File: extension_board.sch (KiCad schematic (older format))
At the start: 39 parts, among them CN1 Conn_02x20_Odd_Even, J1 Screw_Terminal_01x02, J2 Conn_01x02, J3 Conn_01x02, J4 Conn_01x02, J5 Conn_02x03_Odd_Even, J6 Conn_01x02, J7 Conn_02x14_Odd_Even, J8 Conn_02x10_Odd_Even, J9 Conn_02x19_Odd_Even, U1 LM334Z, U2 LM334Z, U3 LM334Z, U4 LM334Z

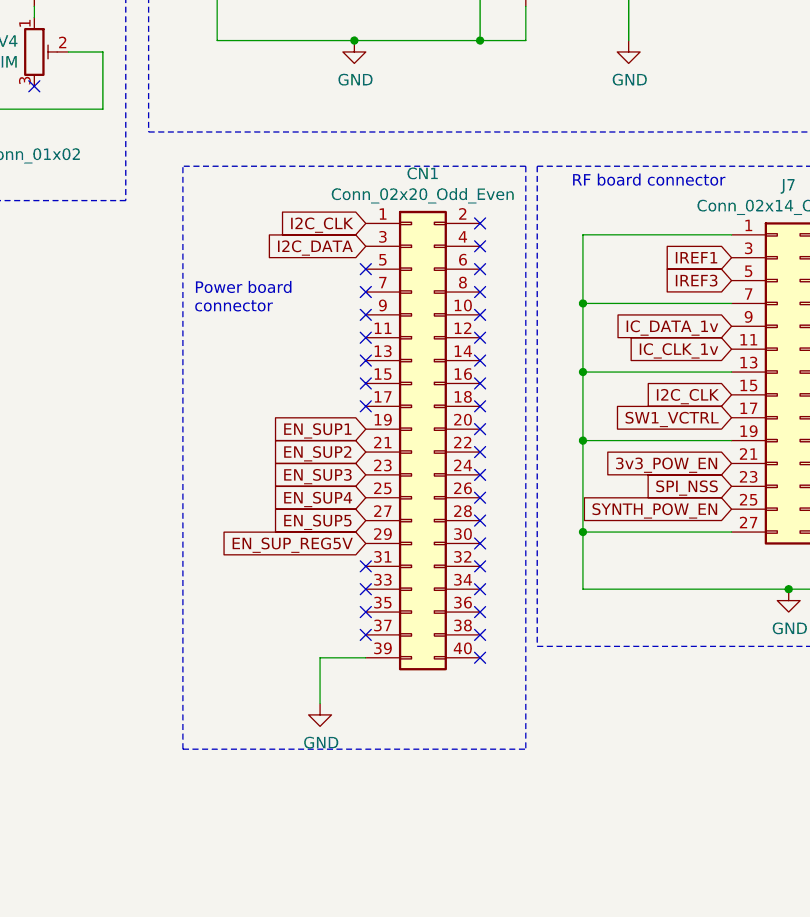
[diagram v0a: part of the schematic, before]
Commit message: gerber files and final files
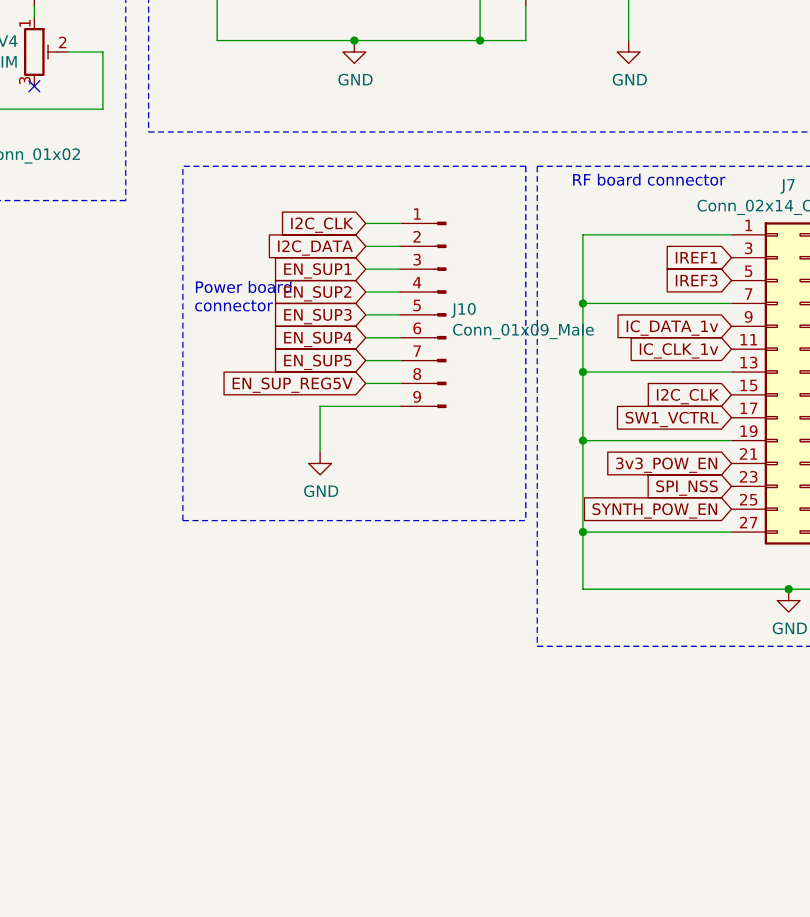
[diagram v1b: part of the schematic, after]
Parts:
- removed CN1: Conn_02x20_Odd_Even, Connector_PinHeader_2.54mm:PinHeader_2x20_P2.54mm_Vertical_SMD, symbol Connector_Generic:Conn_02x20_Odd_Even
- added J10: Conn_01x09_Male, Connector_PinHeader_2.54mm:PinHeader_1x09_P2.54mm_Vertical_SMD_Pin1Left, symbol Connector:Conn_01x09_Male
- J2, J3, J4, J6: footprint Connector_PinHeader_2.54mm:PinHeader_2x01_P2.54mm_Vertical_SMD -> Connector_PinHeader_2.54mm:PinHeader_1x02_P2.54mm_Vertical
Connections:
- net EN_SUP1: now also J10.3 (Pin_3)
- net EN_SUP2: now also J10.4 (Pin_4)
- net EN_SUP3: now also J10.5 (Pin_5)
- net EN_SUP4: now also J10.6 (Pin_6)
- net EN_SUP5: now also J10.7 (Pin_7)
- net EN_SUP_REG5V: now also J10.8 (Pin_8)
- net GND: now also J10.9 (Pin_9)
- net I2C_CLK: now also J10.1 (Pin_1)
- net I2C_DATA: now also J10.2 (Pin_2)
- no-connect marks 58 -> 27
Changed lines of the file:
@@
 1K pot, \nRectangular (3.65mm x 3.00mm x 1.70mm H), \ntop adjust\n
 NoConn ~ 4850 1650
-$Comp
-L Connector_Generic:Conn_02x20_Odd_Even CN1
-U 1 1 6052AEFD
-P 8400 4750
-F 0 "CN1" H 8450 5867 50  0000 C CNN
-F 1 "Conn_02x20_Odd_Even" H 8450 5776 50  0000 C CNN
-F 2 "Connector_PinHeader_2.54mm:PinHeader_2x20_P2.54mm_Vertical_SMD" H 8400 4750 50  0001 C CNN
-F 3 "~" H 8400 4750 50  0001 C CNN
-	1    8400 4750
-	1    0    0    -1
-$EndComp
 Text GLabel 8200 3950 0    50   Input ~ 0
 I2C_DATA
 Text GLabel 8200 3850 0    50   Input ~ 0
 I2C_CLK
-NoConn ~ 8200 4050
-NoConn ~ 8200 4150
-NoConn ~ 8200 4250
-NoConn ~ 8200 4350
-NoConn ~ 8200 4450
-NoConn ~ 8200 4550
-NoConn ~ 8200 4650
-Text GLabel 8200 4750 0    50   Input ~ 0
+Text GLabel 8200 4050 0    50   Input ~ 0
 EN_SUP1
-Text GLabel 8200 4850 0    50   Input ~ 0
+Text GLabel 8200 4150 0    50   Input ~ 0
 EN_SUP2
-Text GLabel 8200 4950 0    50   Input ~ 0
+Text GLabel 8200 4250 0    50   Input ~ 0
 EN_SUP3
-Text GLabel 8200 5050 0    50   Input ~ 0
+Text GLabel 8200 4350 0    50   Input ~ 0
 EN_SUP4
-Text GLabel 8200 5150 0    50   Input ~ 0
+Text GLabel 8200 4450 0    50   Input ~ 0
 EN_SUP5
-Text GLabel 8200 5250 0    50   Input ~ 0
+Text GLabel 8200 4550 0    50   Input ~ 0
 EN_SUP_REG5V
-NoConn ~ 8200 5350
-NoConn ~ 8200 5450
-NoConn ~ 8200 5550
-NoConn ~ 8200 5650
-Wire Wire Line
-	8000 5750 8000 5950
-Wire Wire Line
-	8000 5750 8200 5750
+Wire Wire Line
+	8000 4650 8000 4850
 $Comp
 L power:GND #PWR08
 U 1 1 60545C1E
-P 8000 5950
-F 0 "#PWR08" H 8000 5700 50  0001 C CNN
-F 1 "GND" H 8005 5777 50  0000 C CNN
-F 2 "" H 8000 5950 50  0001 C CNN
-F 3 "" H 8000 5950 50  0001 C CNN
-	1    8000 5950
-	1    0    0    -1
-$EndComp
-NoConn ~ 8700 3850
-NoConn ~ 8700 3950
-NoConn ~ 8700 4050
-NoConn ~ 8700 4150
-NoConn ~ 8700 4250
-NoConn ~ 8700 4350
-NoConn ~ 8700 4450
-NoConn ~ 8700 4550
-NoConn ~ 8700 4650
-NoConn ~ 8700 4750
-NoConn ~ 8700 4850
-NoConn ~ 8700 4950
-NoConn ~ 8700 5050
-NoConn ~ 8700 5150
-NoConn ~ 8700 5250
-NoConn ~ 8700 5350
-NoConn ~ 8700 5450
-NoConn ~ 8700 5550
-NoConn ~ 8700 5650
-NoConn ~ 8700 5750
+P 8000 4850
+F 0 "#PWR08" H 8000 4600 50  0001 C CNN
+F 1 "GND" H 8005 4677 50  0000 C CNN
+F 2 "" H 8000 4850 50  0001 C CNN
+F 3 "" H 8000 4850 50  0001 C CNN
+	1    8000 4850
+	1    0    0    -1
+$EndComp
 Connection ~ 4350 1750
 Wire Wire Line
@@
 Wire Wire Line
 	4350 750  4350 650
-Wire Notes Line
-	8900 3600 8900 6150
-Wire Notes Line
-	7400 6150 7400 3600
 Text Notes 7450 4250 0    50   ~ 0
 Power board \nconnector
@@
 Wire Notes Line
 	8950 3600 11100 3600
-Wire Notes Line
-	7400 6150 8900 6150
 Text GLabel 3850 2250 0    50   Input ~ 0
 VDD
@@
 F 0 "J3" H 4630 1892 50  0000 L CNN
 F 1 "Conn_01x02" H 4630 1801 50  0000 L CNN
-F 2 "Connector_PinHeader_2.54mm:PinHeader_2x01_P2.54mm_Vertical_SMD" H 4550 1900 50  0001 C CNN
+F 2 "Connector_PinHeader_2.54mm:PinHeader_1x02_P2.54mm_Vertical" H 4550 1900 50  0001 C CNN
 F 3 "~" H 4550 1900 50  0001 C CNN
 	1    4550 1900
@@
 F 0 "J2" H 4130 3442 50  0000 L CNN
 F 1 "Conn_01x02" H 4130 3351 50  0000 L CNN
-F 2 "Connector_PinHeader_2.54mm:PinHeader_2x01_P2.54mm_Vertical_SMD" H 4050 3450 50  0001 C CNN
+F 2 "Connector_PinHeader_2.54mm:PinHeader_1x02_P2.54mm_Vertical" H 4050 3450 50  0001 C CNN
 F 3 "~" H 4050 3450 50  0001 C CNN
 	1    4050 3450
@@
 F 0 "J4" H 5380 3442 50  0000 L CNN
 F 1 "Conn_01x02" H 5380 3351 50  0000 L CNN
-F 2 "Connector_PinHeader_2.54mm:PinHeader_2x01_P2.54mm_Vertical_SMD" H 5300 3450 50  0001 C CNN
+F 2 "Connector_PinHeader_2.54mm:PinHeader_1x02_P2.54mm_Vertical" H 5300 3450 50  0001 C CNN
 F 3 "~" H 5300 3450 50  0001 C CNN
 	1    5300 3450
@@
 F 0 "J6" H 6530 3442 50  0000 L CNN
 F 1 "Conn_01x02" H 6530 3351 50  0000 L CNN
-F 2 "Connector_PinHeader_2.54mm:PinHeader_2x01_P2.54mm_Vertical_SMD" H 6450 3450 50  0001 C CNN
+F 2 "Connector_PinHeader_2.54mm:PinHeader_1x02_P2.54mm_Vertical" H 6450 3450 50  0001 C CNN
 F 3 "~" H 6450 3450 50  0001 C CNN
 	1    6450 3450
@@
 	8900 2600 8900 2650
 Connection ~ 8900 2650
+$Comp
+L Connector:Conn_01x09_Male J10
+U 1 1 60D91420
+P 8550 4250
+F 0 "J10" H 8522 4274 50  0000 R CNN
+F 1 "Conn_01x09_Male" H 8522 4183 50  0000 R CNN
+F 2 "Connector_PinHeader_2.54mm:PinHeader_1x09_P2.54mm_Vertical_SMD_Pin1Left" H 8550 4250 50  0001 C CNN
+F 3 "~" H 8550 4250 50  0001 C CNN
+	1    8550 4250
+	-1   0    0    -1
+$EndComp
+Wire Wire Line
+	8200 3850 8350 3850
+Wire Wire Line
+	8350 3950 8200 3950
+Wire Wire Line
+	8200 4050 8350 4050
+Wire Wire Line
+	8200 4150 8350 4150
+Wire Wire Line
+	8200 4250 8350 4250
+Wire Wire Line
+	8200 4350 8350 4350
+Wire Wire Line
+	8200 4450 8350 4450
+Wire Wire Line
+	8200 4550 8350 4550
+Wire Wire Line
+	8000 4650 8350 4650
+Wire Notes Line
+	8900 3600 8900 5150
+Wire Notes Line
+	7400 5150 8900 5150
+Wire Notes Line
+	7400 5150 7400 3600
 $EndSCHEMATC
